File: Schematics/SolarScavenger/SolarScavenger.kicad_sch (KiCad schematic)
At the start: 50 parts, among them J1 SolarConnector, J10 CH1_IN, J11 CH2_IN, J12 CH3_IN, J13 CH4_IN, J14 CH1_OUT, J15 CH2_OUT, J16 CH3_OUT, J17 CH4_OUT, J2 PROGRAMMING, J3 BatteryPack, J4 ESC_PWM_CONTROL, J5 ESC_connector, J6 Micro_SD_Card, J7 RUDDER_POT, J8 THROTTLE_POt, J9 SPARES, Q1 IRLML2502, Q2 IRLML2502, U1 DS18B20, U2 4N25, U3 AP1117-33, U4 ESP32-WROOM-E, U5 INA219AxD

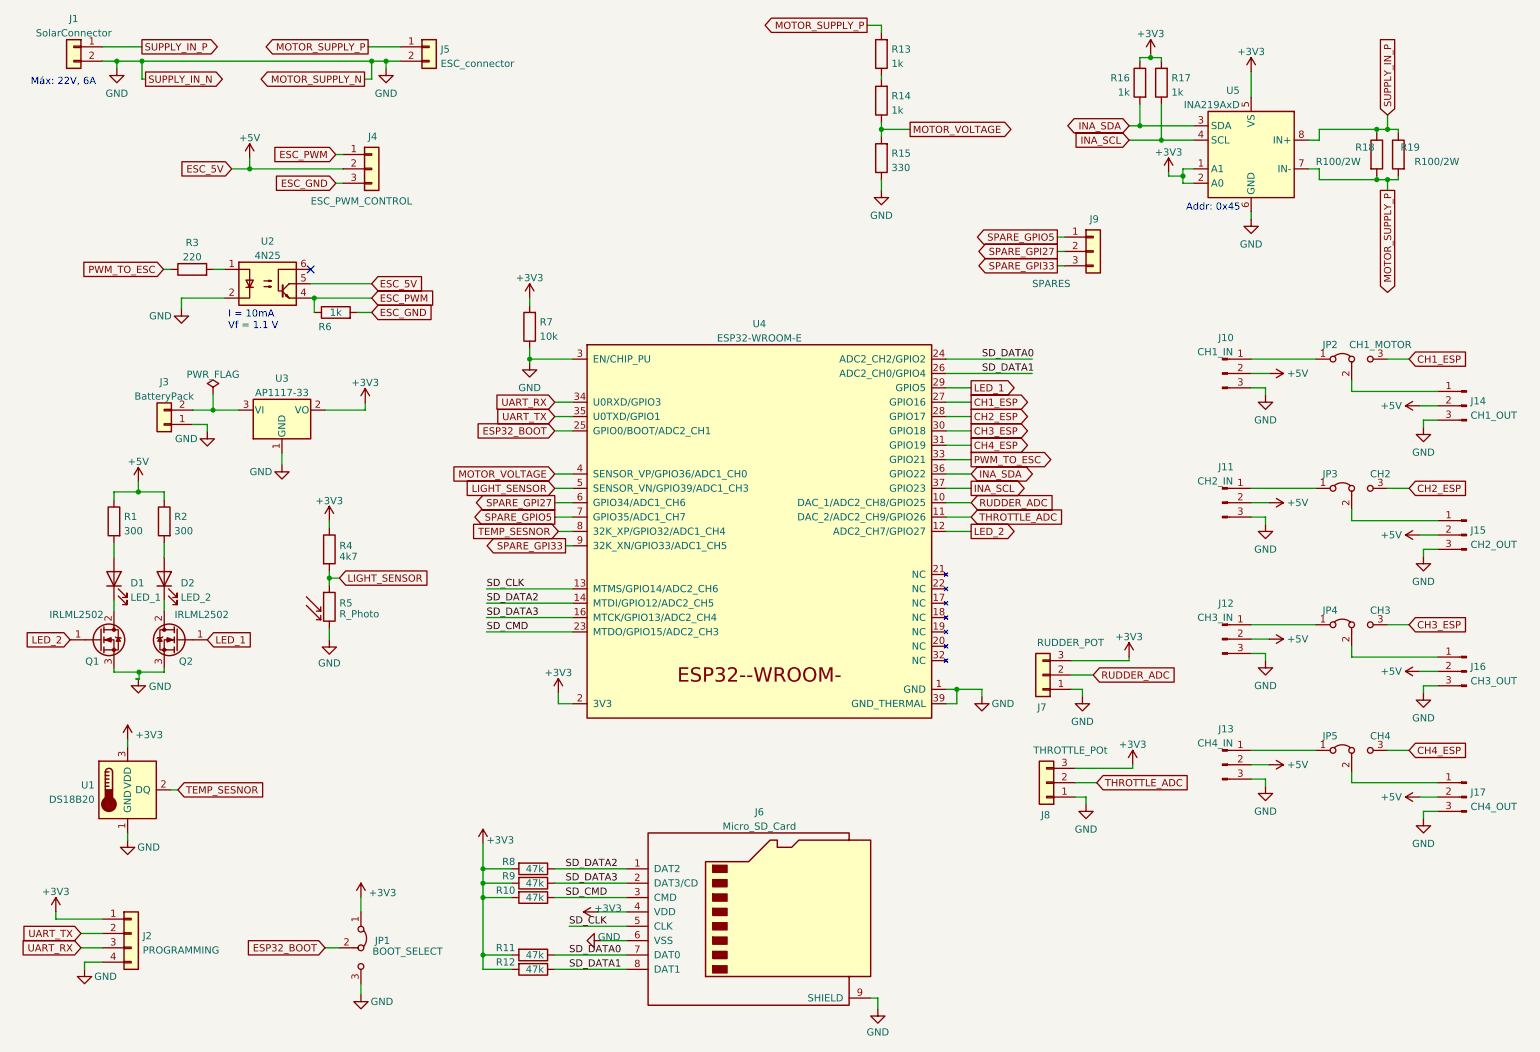
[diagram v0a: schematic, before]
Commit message: PCB final candidate
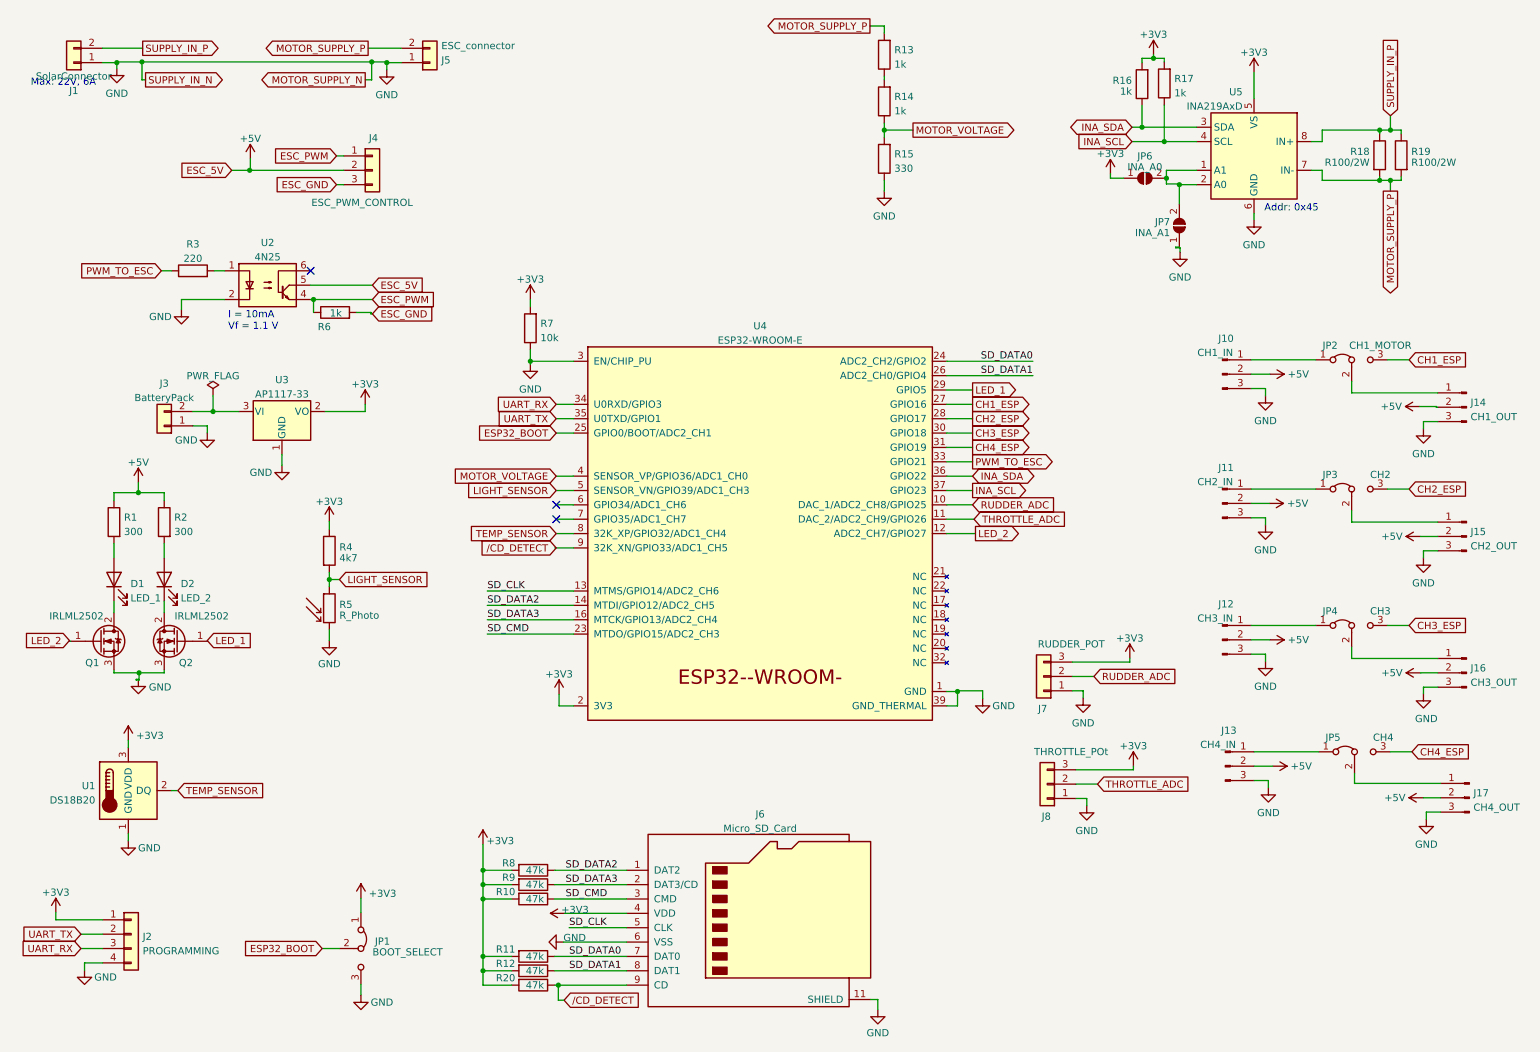
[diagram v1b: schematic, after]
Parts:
- removed J9: SPARES, Connector_PinHeader_2.54mm:PinHeader_1x03_P2.54mm_Vertical, symbol Connector_Generic:Conn_01x03
- added JP6: INA_A0, Jumper:SolderJumper-2_P1.3mm_Open_Pad1.0x1.5mm, symbol Jumper:SolderJumper_2_Open
- added JP7: INA_A1, Jumper:SolderJumper-2_P1.3mm_Open_Pad1.0x1.5mm, symbol Jumper:SolderJumper_2_Open
- added R20: 47k, Resistor_SMD:R_1206_3216Metric_Pad1.30x1.75mm_HandSolder, symbol Device:R
- D1, D2: footprint LED_THT:LED_D5.0mm -> LED_SMD:LED_1210_3225Metric_Pad1.42x2.65mm_HandSolder
- R10, R11, R12, R13, R14, R15, R16, R17, R4, R7, R8, R9: footprint Resistor_SMD:R_1020_2550Metric_Pad1.33x5.20mm_HandSolder -> Resistor_SMD:R_1206_3216Metric_Pad1.30x1.75mm_HandSolder
- U3: footprint Package_TO_SOT_SMD:SOT-223-3_TabPin2 -> Package_TO_SOT_THT:TO-220-3_Vertical
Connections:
- net +3V3: now also R16.2, JP6.1 (A), R20.2; no longer R16.1, U5.1 (A1), U5.2 (A0)
- net GND: now also J1.1 (Pin_1), J5.1 (Pin_1), J6.11 (SHIELD), JP7.1 (A); no longer J1.2 (Pin_2), J5.2 (Pin_2), J6.9 (SHIELD)
- net INA_SDA: now also R16.1; no longer R16.2
- net MOTOR_SUPPLY_P: now also J5.2 (Pin_2); no longer J5.1 (Pin_1)
- net SUPPLY_IN_P: now also J1.2 (Pin_2); no longer J1.1 (Pin_1)
- net SPARE_GPI27: no longer names the net of U4.6 (GPIO34/ADC1_CH6)
- net SPARE_GPI33 renamed /CD_DETECT
- net /CD_DETECT: now also J6.9 (CD), R20.1
- net SPARE_GPIO5: no longer names the net of U4.7 (GPIO35/ADC1_CH7)
- net TEMP_SESNOR renamed TEMP_SENSOR
- new net: JP6.2 (B), JP7.2 (B), U5.1 (A1), U5.2 (A0)
- no-connect marks 1 -> 3
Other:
- moved on the sheet: J1, J13, J17, JP5, R13, R14, R15, R17, R18, R19, U5
